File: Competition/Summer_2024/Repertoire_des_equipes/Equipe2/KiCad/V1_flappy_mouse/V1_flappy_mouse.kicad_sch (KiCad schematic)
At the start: 0 parts

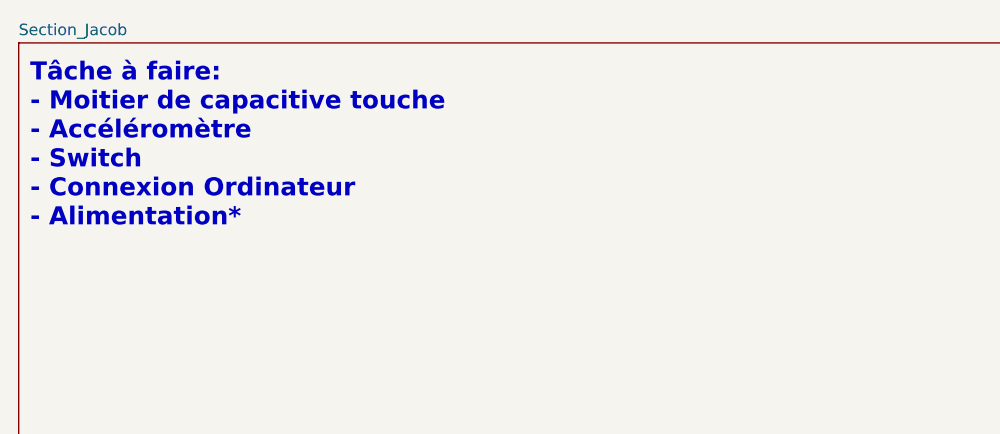
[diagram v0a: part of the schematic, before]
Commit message: Push des changements fait
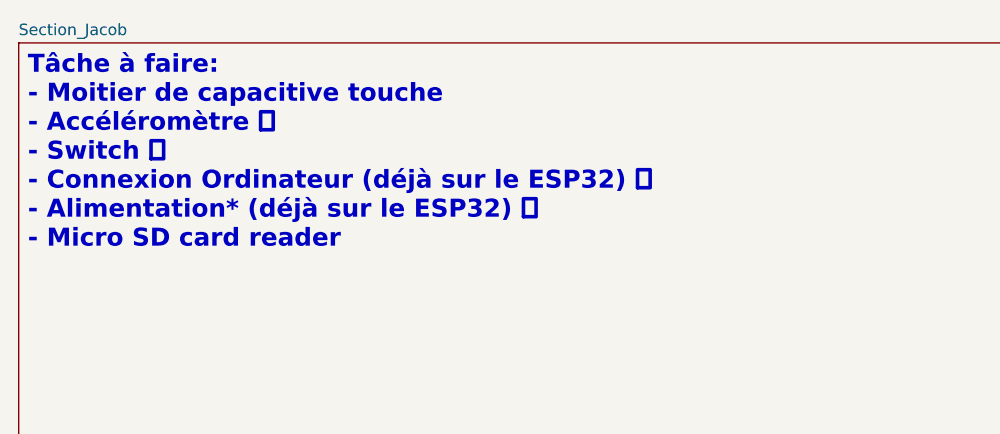
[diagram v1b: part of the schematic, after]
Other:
- note added: "Tâche à faire: - Moitier de capacitive touche - Accéléromètre ❎ - Switch ❎ - Connexion Ordinateur (déjà sur le ESP32) ❎ - Alimentation* (déjà sur le ESP32) ❎ - Micro SD card reader"
- note removed: "Tâche à faire: - Moitier de capacitive touche - Accéléromètre - Switch - Connexion Ordinateur - Alimentation*"
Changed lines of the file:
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@@
 		)
 	)
-	(text "Tâche à faire:\n- Moitier de capacitive touche\n- Accéléromètre\n- Switch\n- Connexion Ordinateur\n- Alimentation*"
+	(text "Tâche à faire:\n- Moitier de capacitive touche \n- Accéléromètre ❎\n- Switch ❎ \n- Connexion Ordinateur (déjà sur le ESP32) ❎\n- Alimentation* (déjà sur le ESP32) ❎\n- Micro SD card reader"
 		(exclude_from_sim no)
-		(at 15.24 26.67 0)
+		(at 14.986 27.432 0)
 		(effects
 			(font
